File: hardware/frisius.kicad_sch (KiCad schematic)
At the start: 0 parts

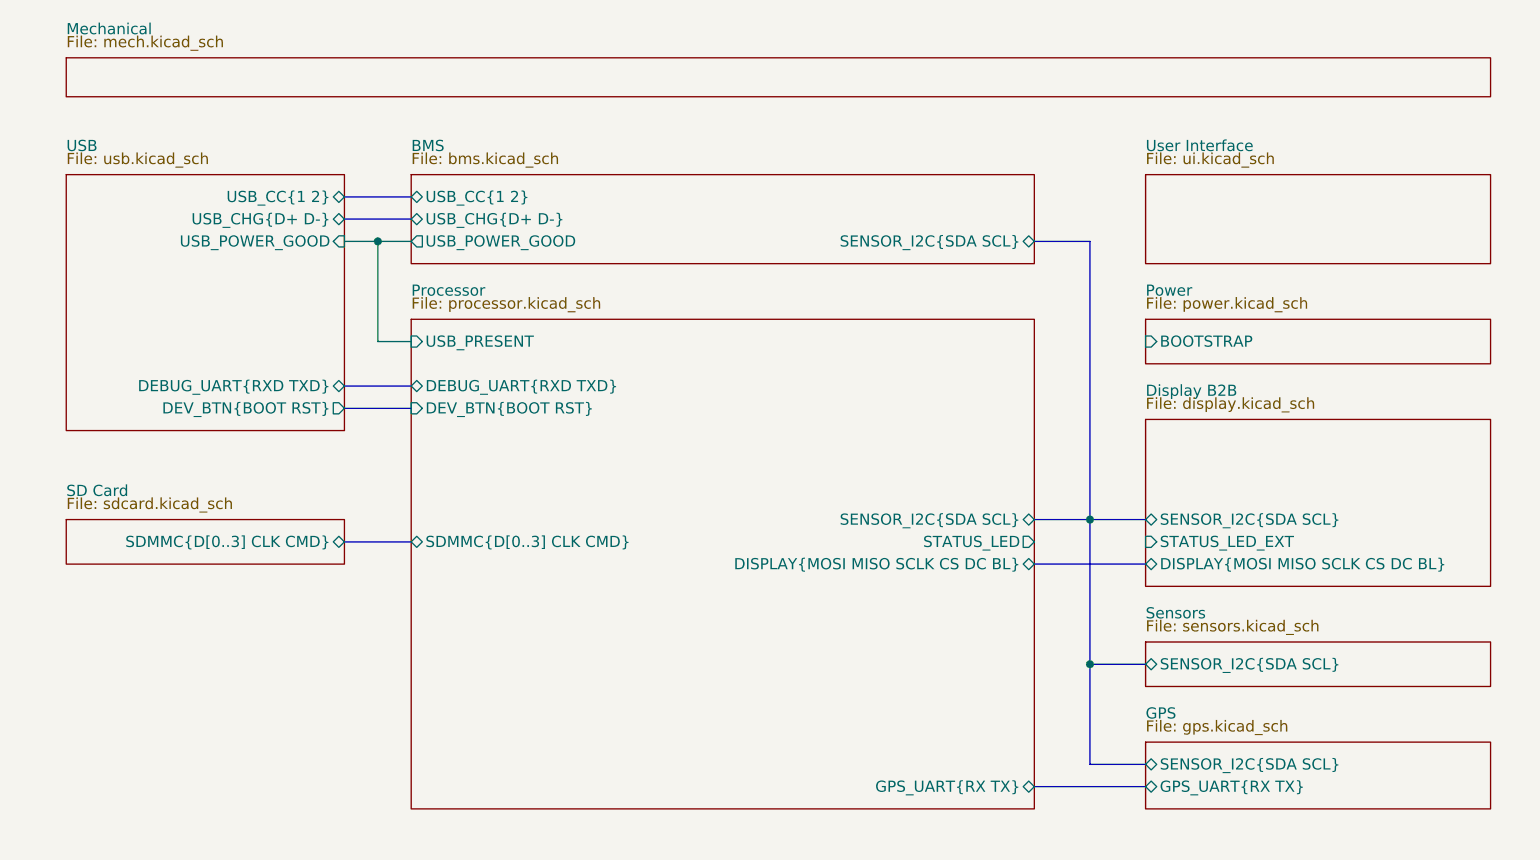
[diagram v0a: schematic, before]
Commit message: Updates
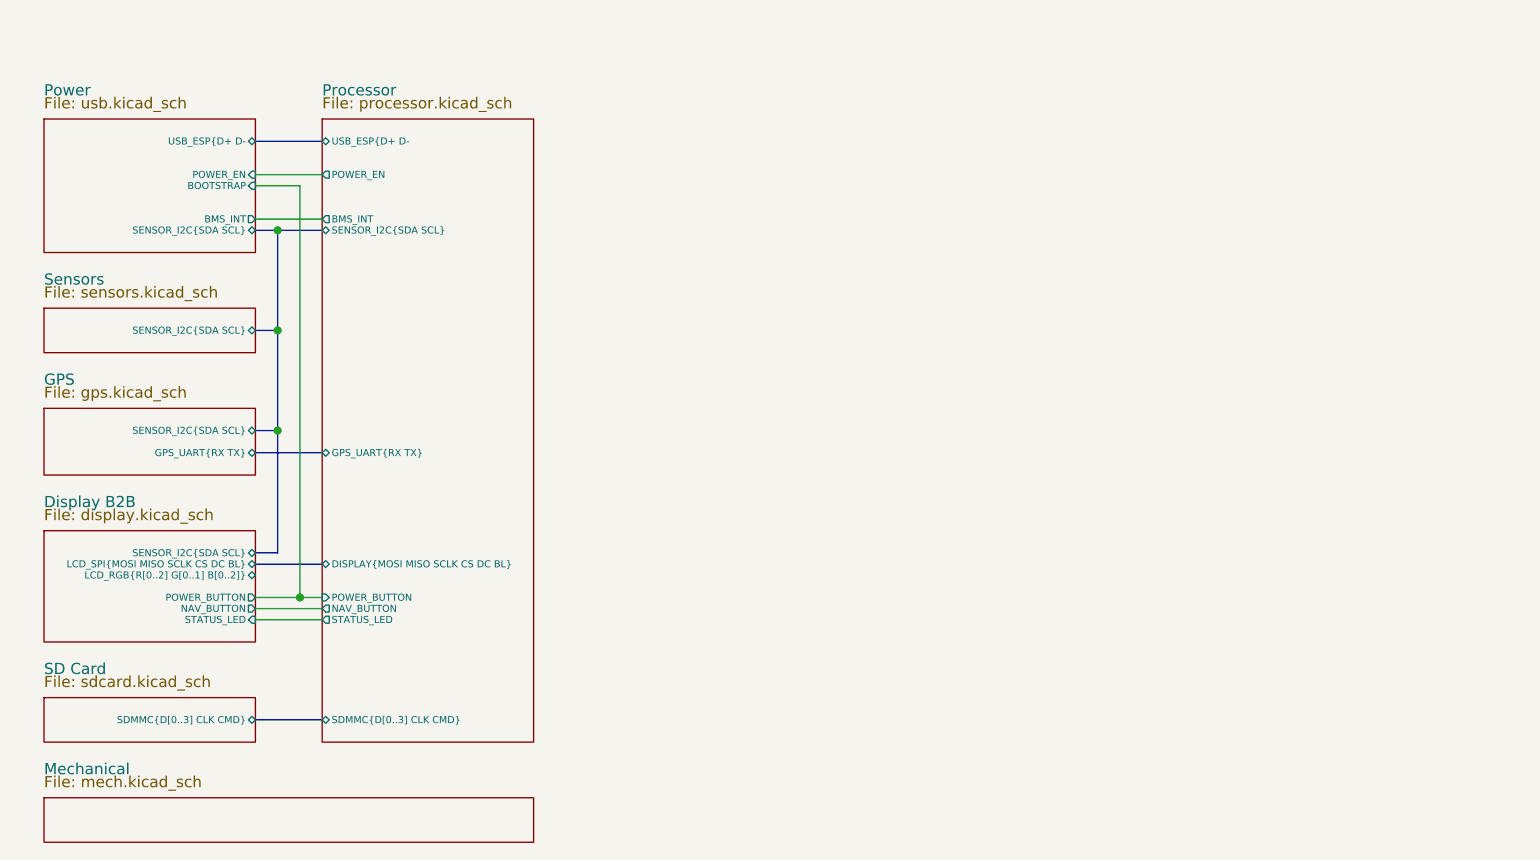
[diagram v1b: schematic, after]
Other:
- removed sheet BMS
- removed sheet USB
- removed sheet User Interface
- sheet Display B2B ports: added LCD_RGB{R[0..2] G[0..1] B[0..2]}, LCD_SPI{MOSI MISO SCLK CS DC BL}, NAV_BUTTON, POWER_BUTTON, STATUS_LED; removed DISPLAY{MOSI MISO SCLK CS DC BL}, STATUS_LED_EXT
- sheet Power: file power.kicad_sch -> usb.kicad_sch
- sheet Power ports: added BMS_INT, POWER_EN, SENSOR_I2C{SDA SCL}, USB_ESP{D+ D-; removed none
- sheet Processor ports: added BMS_INT, NAV_BUTTON, POWER_BUTTON, POWER_EN, USB_ESP{D+ D-; removed DEBUG_UART{RXD TXD}, DEV_BTN{BOOT RST}, USB_PRESENT
